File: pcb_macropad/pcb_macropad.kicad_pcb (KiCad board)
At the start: 2 copper layers, 57.2 x 73 mm, 26 parts, among them J1 OLED_128x32, SW1 RotaryEncoder_Switch, U1 Arduino_Pro_Micro

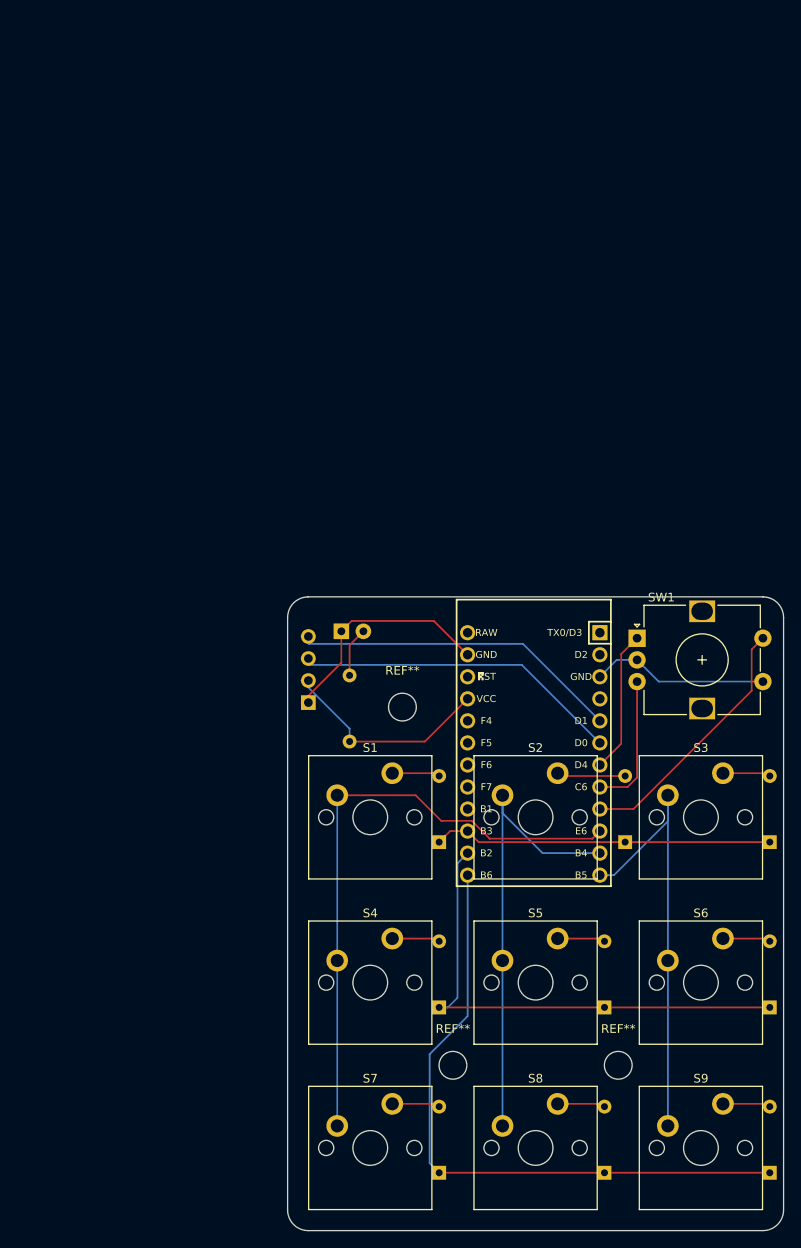
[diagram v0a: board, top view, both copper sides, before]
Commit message: Updates
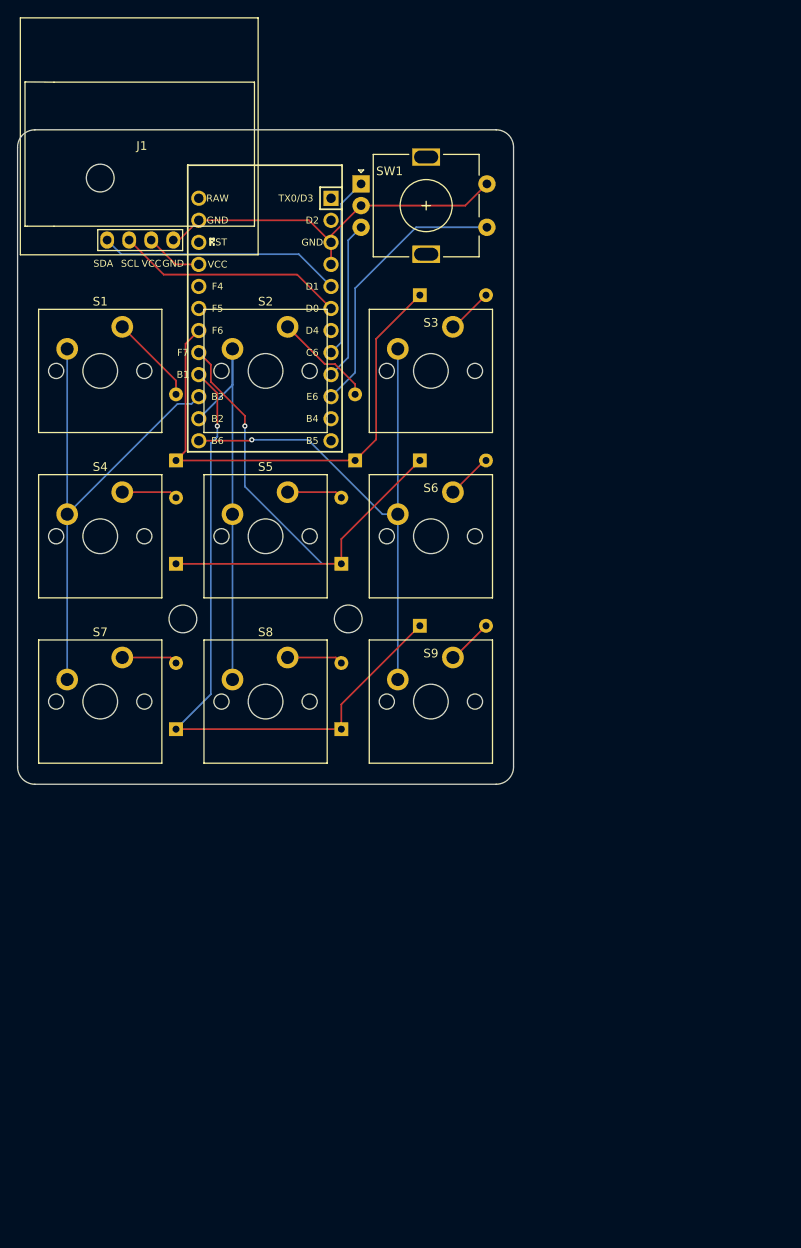
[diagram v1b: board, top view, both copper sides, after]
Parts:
- removed D10: LED, LED_THT:LED_D5.0mm
- removed R1: R330, Resistor_THT:R_Axial_DIN0207_L6.3mm_D2.5mm_P7.62mm_Horizontal
- removed the REF** at (125.4, 141.3)
- removed the REF** at (100.5, 100.0)
- removed the REF** at (106.4, 141.3)
- added REF**: MountingHole_3.2mm_M3, MountingHole:MountingHole_3.2mm_M3, F.Cu at (65.7, 39.1)
- added REF**: MountingHole_3.2mm_M3, MountingHole:MountingHole_3.2mm_M3, F.Cu at (94.3, 89.9)
- added REF**: MountingHole_3.2mm_M3, MountingHole:MountingHole_3.2mm_M3, F.Cu at (75.2, 89.9)
- J1: value OLED_128x32 -> OLED_128x64; footprint ScottoKeebs_Components:OLED_128x32 -> SSD1306:128x64OLED
- SW1: footprint Rotary_Encoder:RotaryEncoder_Alps_EC12E-Switch_Vertical_H20mm -> Rotary_Encoder:RotaryEncoder_Alps_EC11E-Switch_Vertical_H20mm
- moved D6 74.8 mm to (102.6, 71.6), turned to 0 degrees
- moved D3 74.8 mm to (102.6, 52.5), turned to 0 degrees
- moved D9 74.8 mm to (102.6, 90.6), turned to 0 degrees
- moved SW1 61.3 mm to (95.8, 39.7)
- moved S1 60.1 mm to (65.7, 61.3)
- moved S2 60.1 mm to (84.8, 61.3)
- moved S7 60.1 mm to (65.7, 99.4)
- moved S8 60.1 mm to (84.8, 99.4)
- moved S3 60.1 mm to (103.8, 61.3)
- moved S9 60.1 mm to (103.8, 99.4)
- moved S4 60.1 mm to (65.7, 80.3)
- moved S5 60.1 mm to (84.8, 80.3)
- moved S6 60.1 mm to (103.8, 80.3)
- moved D4 59.4 mm to (74.5, 83.5)
- moved D5 59.4 mm to (93.5, 83.5)
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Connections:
- net +5V renamed VCC
- D1 pad 1: Row1 -> Row 1
- D2 pad 1: Row1 -> Row 1
- D3 pad 1: Row1 -> Row 1
- D4 pad 1: Row2 -> Row 2
- D5 pad 1: Row2 -> Row 2
- D6 pad 1: Row2 -> Row 2
- D7 pad 1: Row3 -> Row 3
- D8 pad 1: Row3 -> Row 3
- D9 pad 1: Row3 -> Row 3
- S1 pad 1: Col1 -> Column 1
- S2 pad 1: Col2 -> Column 2
- S3 pad 1: Col3 -> Column 3
- S4 pad 1: Col1 -> Column 1
- S5 pad 1: Col2 -> Column 2
- S6 pad 1: Col3 -> Column 3
- S7 pad 1: Col1 -> Column 1
- S8 pad 1: Col2 -> Column 2
- S9 pad 1: Col3 -> Column 3
- U1 pad 10: Col1 -> EncoderSW
- U1 pad 11: Col2 -> unconnected-(U1-8/PB4-Pad11)
- U1 pad 12: Col3 -> unconnected-(U1-9/PB5-Pad12)
- U1 pad 13: Row3 -> Column 3
- U1 pad 14: Row2 -> Column 2
- U1 pad 15: Row1 -> Column 1
- U1 pad 16: unconnected-(U1-15/PB1-Pad16) -> Row 3
- U1 pad 17: unconnected-(U1-A0/PF7-Pad17) -> Row 2
- U1 pad 18: unconnected-(U1-A1/PF6-Pad18) -> Row 1
- U1 pad 7: EncoderA -> unconnected-(U1-4/PD4-Pad7)
- U1 pad 8: EncoderB -> EncoderA
- U1 pad 9: EncoderSW -> EncoderB
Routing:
- net Row 3: track 0.00 -> 78.4 mm, vias 0 -> 1
- net Row3: track 74.7 -> 0.00 mm
- net Col1: track 70.8 -> 0.00 mm
- net Row 2: track 0.00 -> 67.1 mm, vias 0 -> 1
- net Column 3: track 0.00 -> 64.6 mm, vias 0 -> 1
- net Column 1: track 0.00 -> 58.9 mm
- net Row 1: track 0.00 -> 58.8 mm
- net Row2: track 57.8 -> 0.00 mm
- net Col2: track 53.3 -> 0.00 mm
- net Col3: track 51.5 -> 0.00 mm
- net Column 2: track 0.00 -> 47.8 mm
- net Row1: track 39.2 -> 0.00 mm
- net VCC: track 25.0 -> 6.64 mm
- net SCL: track 38.4 -> 26.5 mm
- net SDA: track 38.4 -> 28.0 mm
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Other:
- board size 57.2 x 73 mm -> 57.1 x 75.4 mm
- board text added: "GND"
- board text added: "SCL"
- board text added: "SDA"
- board text added: "VCC"
